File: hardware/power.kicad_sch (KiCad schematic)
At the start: 2 parts, among them P8 Conn_01x06, P9 Conn_01x06

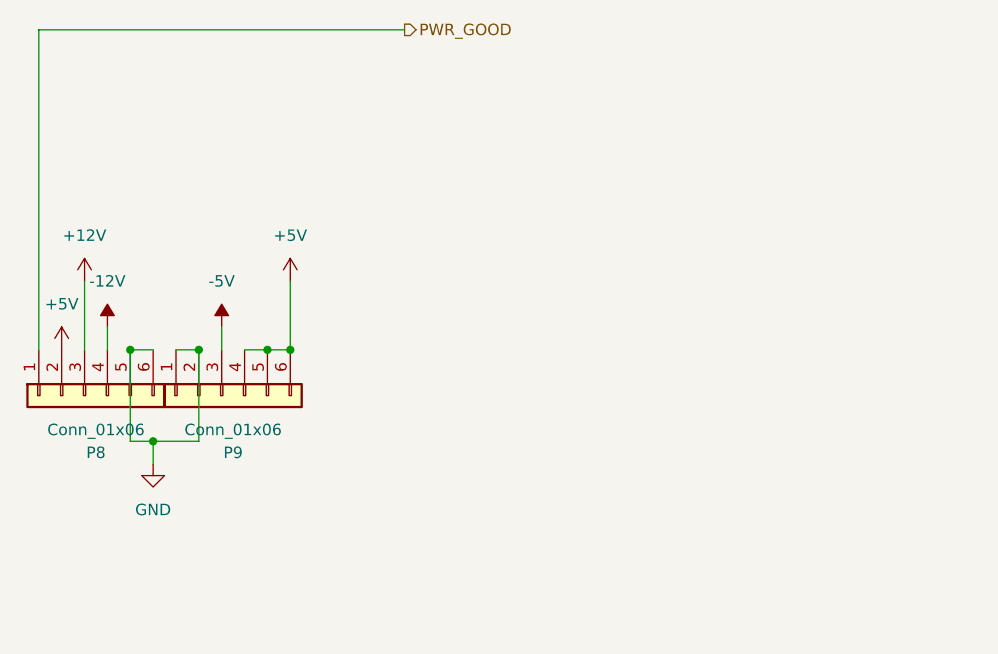
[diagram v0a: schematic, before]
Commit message: getting closer
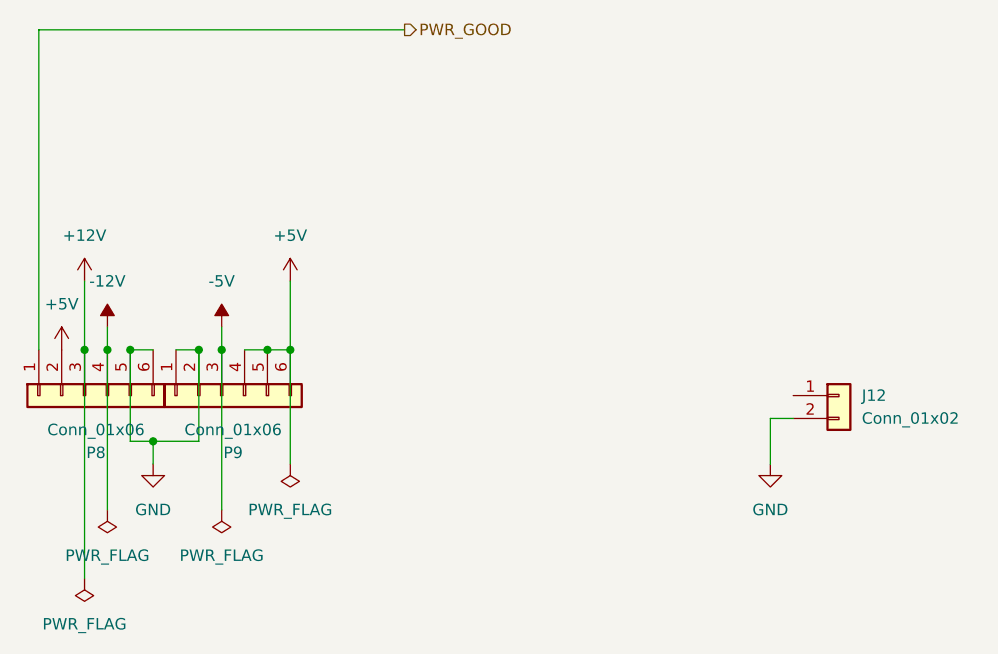
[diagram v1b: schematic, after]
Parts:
- added J12: Conn_01x02, symbol Connector_Generic:Conn_01x02
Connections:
- net GND: now also J12.2 (Pin_2)
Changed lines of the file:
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@@
 (kicad_sch (version 20230121) (generator eeschema)
   (paper "A4")
+  (junction (at 127 88.9) (diameter 0) (color 0 0 0 0)
+  )
   (junction (at 132.08 88.9) (diameter 0) (color 0 0 0 0)
   )
+  (junction (at 111.76 88.9) (diameter 0) (color 0 0 0 0)
+  )
   (junction (at 116.84 88.9) (diameter 0) (color 0 0 0 0)
   )
@@
   (junction (at 124.46 88.9) (diameter 0) (color 0 0 0 0)
   )
+  (junction (at 114.3 88.9) (diameter 0) (color 0 0 0 0)
+  )
   (wire (pts (xy 119.38 99.06) (xy 116.84 99.06))
     (stroke (width 0) (type default))
@@
     (stroke (width 0) (type default))
   )
+  (wire (pts (xy 190.5 96.52) (xy 187.96 96.52))
+    (stroke (width 0) (type default))
+  )
   (wire (pts (xy 116.84 88.9) (xy 116.84 99.06))
     (stroke (width 0) (type default))
@@
     (stroke (width 0) (type default))
   )
+  (wire (pts (xy 114.3 88.9) (xy 114.3 106.68))
+    (stroke (width 0) (type default))
+  )
   (wire (pts (xy 127 86.36) (xy 127 88.9))
     (stroke (width 0) (type default))
@@
     (stroke (width 0) (type default))
   )
+  (wire (pts (xy 134.62 88.9) (xy 134.62 101.6))
+    (stroke (width 0) (type default))
+  )
   (wire (pts (xy 132.08 88.9) (xy 129.54 88.9))
     (stroke (width 0) (type default))
@@
     (stroke (width 0) (type default))
   )
+  (wire (pts (xy 127 88.9) (xy 127 106.68))
+    (stroke (width 0) (type default))
+  )
+  (wire (pts (xy 187.96 96.52) (xy 187.96 101.6))
+    (stroke (width 0) (type default))
+  )
   (wire (pts (xy 124.46 99.06) (xy 119.38 99.06))
+    (stroke (width 0) (type default))
+  )
+  (wire (pts (xy 111.76 88.9) (xy 111.76 114.3))
     (stroke (width 0) (type default))
   )
@@
         (path "/3006deba-2100-40f8-9f39-987a5c2c14c7/f8ecdba8-12ed-4532-a81b-3b086d58d046"
           (reference "#PWR013") (unit 1)
+        )
+      )
+    )
+  )
+  (symbol (lib_id "Connector_Generic:Conn_01x02") (at 195.58 93.98 0) (unit 1)
+    (in_bom yes) (on_board yes) (dnp no) (fields_autoplaced)
+    (property "Reference" "J12" (at 198.12 93.98 0)
+      (effects (font (size 1.27 1.27)) (justify left))
+    )
+    (property "Value" "Conn_01x02" (at 198.12 96.52 0)
+      (effects (font (size 1.27 1.27)) (justify left))
+    )
+    (property "Footprint" "" (at 195.58 93.98 0)
+      (effects (font (size 1.27 1.27)) hide)
+    )
+    (property "Datasheet" "~" (at 195.58 93.98 0)
+      (effects (font (size 1.27 1.27)) hide)
+    )
+    (pin "2")
+    (pin "1")
+    (instances
+      (project "68040pc"
+        (path "/3006deba-2100-40f8-9f39-987a5c2c14c7/f8ecdba8-12ed-4532-a81b-3b086d58d046"
+          (reference "J12") (unit 1)
         )
       )
@@
     )
   )
+  (symbol (lib_id "power:PWR_FLAG") (at 114.3 106.68 0) (mirror x) (unit 1)
+    (in_bom yes) (on_board yes) (dnp no) (fields_autoplaced)
+    (property "Reference" "#FLG04" (at 114.3 108.585 0)
+      (effects (font (size 1.27 1.27)) hide)
+    )
+    (property "Value" "PWR_FLAG" (at 114.3 111.76 0)
+      (effects (font (size 1.27 1.27)))
+    )
+    (property "Footprint" "" (at 114.3 106.68 0)
+      (effects (font (size 1.27 1.27)) hide)
+    )
+    (property "Datasheet" "~" (at 114.3 106.68 0)
+      (effects (font (size 1.27 1.27)) hide)
+    )
+    (pin "1")
+    (instances
+      (project "68040pc"
+        (path "/3006deba-2100-40f8-9f39-987a5c2c14c7/f8ecdba8-12ed-4532-a81b-3b086d58d046"
+          (reference "#FLG04") (unit 1)
+        )
+      )
+    )
+  )
   (symbol (lib_id "power:GND") (at 119.38 101.6 0) (unit 1)
     (in_bom yes) (on_board yes) (dnp no) (fields_autoplaced)
@@
         (path "/3006deba-2100-40f8-9f39-987a5c2c14c7/f8ecdba8-12ed-4532-a81b-3b086d58d046"
           (reference "#PWR014") (unit 1)
+        )
+      )
+    )
+  )
+  (symbol (lib_id "power:PWR_FLAG") (at 134.62 101.6 0) (mirror x) (unit 1)
+    (in_bom yes) (on_board yes) (dnp no) (fields_autoplaced)
+    (property "Reference" "#FLG02" (at 134.62 103.505 0)
+      (effects (font (size 1.27 1.27)) hide)
+    )
+    (property "Value" "PWR_FLAG" (at 134.62 106.68 0)
+      (effects (font (size 1.27 1.27)))
+    )
+    (property "Footprint" "" (at 134.62 101.6 0)
+      (effects (font (size 1.27 1.27)) hide)
+    )
+    (property "Datasheet" "~" (at 134.62 101.6 0)
+      (effects (font (size 1.27 1.27)) hide)
+    )
+    (pin "1")
+    (instances
+      (project "68040pc"
+        (path "/3006deba-2100-40f8-9f39-987a5c2c14c7/f8ecdba8-12ed-4532-a81b-3b086d58d046"
+          (reference "#FLG02") (unit 1)
+        )
+      )
+    )
+  )
+  (symbol (lib_id "power:PWR_FLAG") (at 111.76 114.3 0) (mirror x) (unit 1)
+    (in_bom yes) (on_board yes) (dnp no) (fields_autoplaced)
+    (property "Reference" "#FLG01" (at 111.76 116.205 0)
+      (effects (font (size 1.27 1.27)) hide)
+    )
+    (property "Value" "PWR_FLAG" (at 111.76 119.38 0)
+      (effects (font (size 1.27 1.27)))
+    )
+    (property "Footprint" "" (at 111.76 114.3 0)
+      (effects (font (size 1.27 1.27)) hide)
+    )
+    (property "Datasheet" "~" (at 111.76 114.3 0)
+      (effects (font (size 1.27 1.27)) hide)
+    )
+    (pin "1")
+    (instances
+      (project "68040pc"
+        (path "/3006deba-2100-40f8-9f39-987a5c2c14c7/f8ecdba8-12ed-4532-a81b-3b086d58d046"
+          (reference "#FLG01") (unit 1)
         )
       )
@@
     )
   )
+  (symbol (lib_id "power:PWR_FLAG") (at 127 106.68 0) (mirror x) (unit 1)
+    (in_bom yes) (on_board yes) (dnp no) (fields_autoplaced)
+    (property "Reference" "#FLG03" (at 127 108.585 0)
+      (effects (font (size 1.27 1.27)) hide)
+    )
+    (property "Value" "PWR_FLAG" (at 127 111.76 0)
+      (effects (font (size 1.27 1.27)))
+    )
+    (property "Footprint" "" (at 127 106.68 0)
+      (effects (font (size 1.27 1.27)) hide)
+    )
+    (property "Datasheet" "~" (at 127 106.68 0)
+      (effects (font (size 1.27 1.27)) hide)
+    )
+    (pin "1")
+    (instances
+      (project "68040pc"
+        (path "/3006deba-2100-40f8-9f39-987a5c2c14c7/f8ecdba8-12ed-4532-a81b-3b086d58d046"
+          (reference "#FLG03") (unit 1)
+        )
+      )
+    )
+  )
   (symbol (lib_id "power:+5V") (at 109.22 88.9 0) (unit 1)
     (in_bom yes) (on_board yes) (dnp no) (fields_autoplaced)
@@
         )
       )
+    )
+  )
+  (symbol (lib_id "power:GND") (at 187.96 101.6 0) (unit 1)
+    (in_bom yes) (on_board yes) (dnp no) (fields_autoplaced)
+    (property "Reference" "#PWR014" (at 187.96 107.95 0)
+      (effects (font (size 1.27 1.27)) hide)
+    )
+    (property "Value" "GND" (at 187.96 106.68 0)
+      (effects (font (size 1.27 1.27)))
+    )
+    (property "Footprint" "" (at 187.96 101.6 0)
+      (effects (font (size 1.27 1.27)) hide)
+    )
+    (property "Datasheet" "" (at 187.96 101.6 0)
+      (effects (font (size 1.27 1.27)) hide)
+    )
+    (pin "1")
+    (instances
+      (project "68040pc"
+        (path "/3006deba-2100-40f8-9f39-987a5c2c14c7"
+          (reference "#PWR014") (unit 1)
+        )
+        (path "/3006deba-2100-40f8-9f39-987a5c2c14c7/f8ecdba8-12ed-4532-a81b-3b086d58d046"
+          (reference "#PWR032") (unit 1)
+        )
+      )
